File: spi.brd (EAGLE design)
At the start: 34 x 33 mm, 5 parts, among them IC2 25AA080SN, IC3 25AA080P, X1 2510-

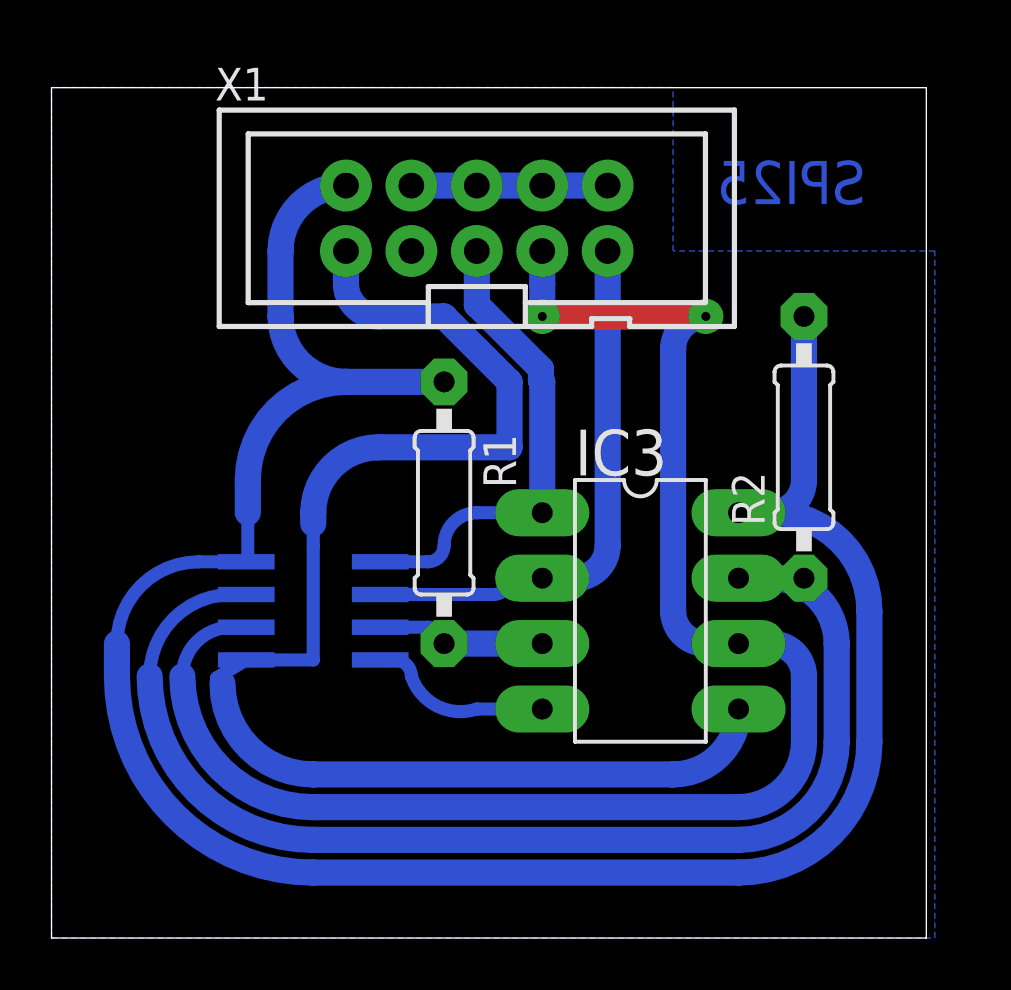
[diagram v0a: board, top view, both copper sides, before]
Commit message: Fixed polygon
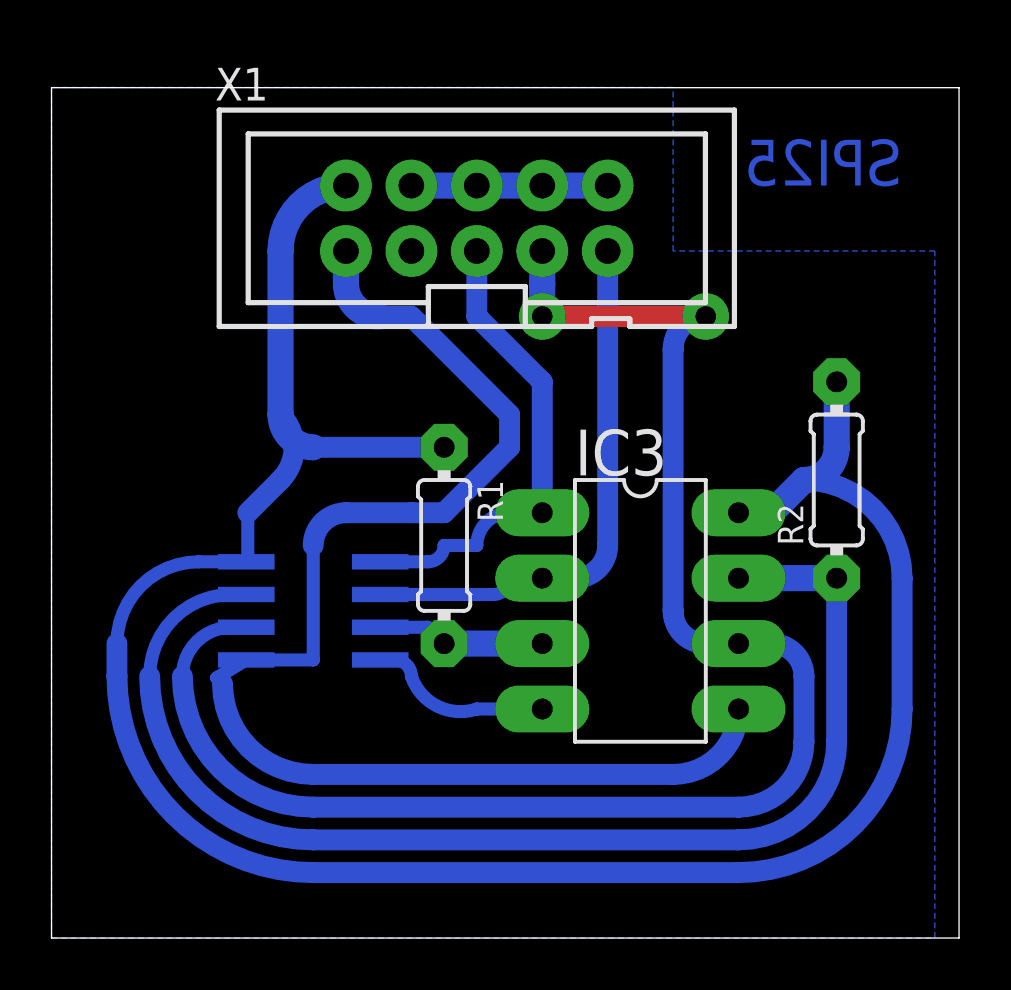
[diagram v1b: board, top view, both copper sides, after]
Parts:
- R1, R2: value 330 -> (none); device eagle-ltspice:0207/10 -> eagle-ltspice:0204/7
- moved R2 1.80 mm to (39.4, 34.3)
- moved R1 1.27 mm to (24.1, 31.8)
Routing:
- net SI: track 52.9 -> 51.4 mm
- net HOLD: track 47.2 -> 46.1 mm
- net VCC: track 84.1 -> 84.8 mm
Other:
- board size 34 x 33 mm -> 35.2 x 33 mm
